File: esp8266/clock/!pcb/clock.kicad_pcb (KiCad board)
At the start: 2 copper layers, 45.2 x 57 mm, 17 parts, among them J1 GPIO, U3 BME280, U4 OLED, U5 LED, U6 SPARE

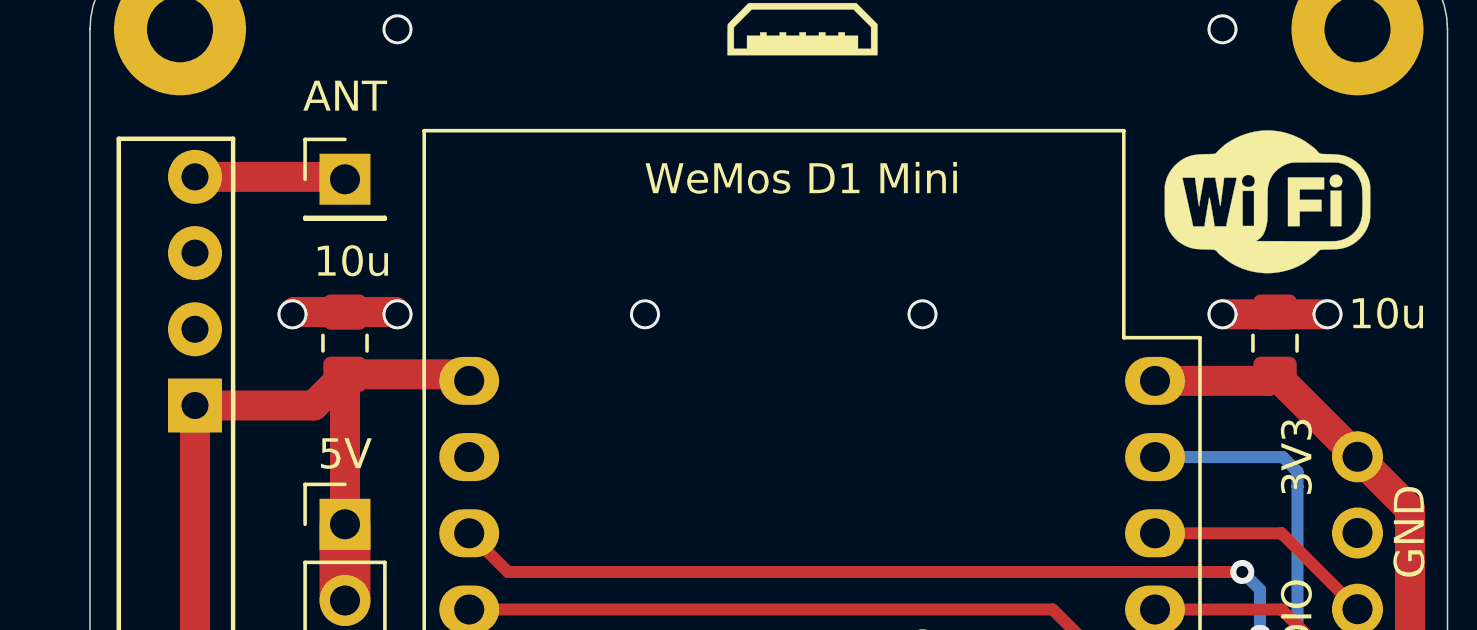
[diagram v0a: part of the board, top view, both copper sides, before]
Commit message: clock: Almost ready
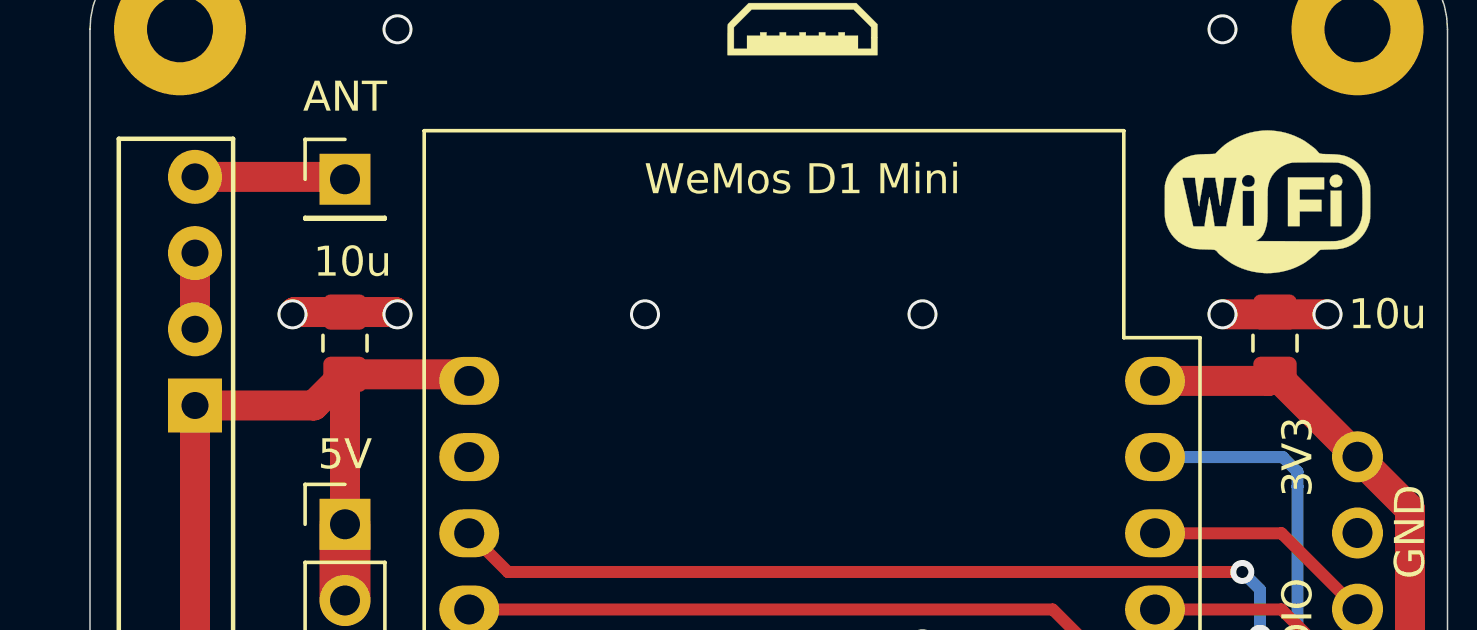
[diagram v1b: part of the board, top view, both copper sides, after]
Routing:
- net GND: track 13.1 -> 15.6 mm
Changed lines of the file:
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@@
     (thickness 1.6)
     (drawings 23)
-    (tracks 111)
+    (tracks 112)
     (zones 0)
     (modules 17)
@@
       (outputformat 1)
       (mirror false)
-      (drillshape 1)
+      (drillshape 0)
       (scaleselection 1)
-      (outputdirectory ""))
+      (outputdirectory "gerbs/"))
   )
   (net 0 "")
@@
       (effects (font (size 0.5 0.5) (thickness 0.08)))
     )
-    (pad 1 smd roundrect (at -1.0375 0 90) (size 1.175 1.45) (layers F.Cu F.Paste F.Mask) (roundrect_rratio 0.212766)
+    (pad 1 smd roundrect (at -1.0375 0 90) (size 1.175 1.45) (layers F.Cu F.Paste F.Mask) (roundrect_rratio 0.2127659574468085)
       (net 1 +5V))
-    (pad 2 smd roundrect (at 1.0375 0 90) (size 1.175 1.45) (layers F.Cu F.Paste F.Mask) (roundrect_rratio 0.212766)
+    (pad 2 smd roundrect (at 1.0375 0 90) (size 1.175 1.45) (layers F.Cu F.Paste F.Mask) (roundrect_rratio 0.2127659574468085)
       (net 2 GND))
     (model ${KISYS3DMOD}/Capacitor_SMD.3dshapes/C_0805_2012Metric.wrl
@@
       (effects (font (size 0.5 0.5) (thickness 0.08)))
     )
-    (pad 2 smd roundrect (at 1.0375 0 270) (size 1.175 1.45) (layers F.Cu F.Paste F.Mask) (roundrect_rratio 0.212766)
+    (pad 2 smd roundrect (at 1.0375 0 270) (size 1.175 1.45) (layers F.Cu F.Paste F.Mask) (roundrect_rratio 0.2127659574468085)
       (net 3 +3V3))
-    (pad 1 smd roundrect (at -1.0375 0 270) (size 1.175 1.45) (layers F.Cu F.Paste F.Mask) (roundrect_rratio 0.212766)
+    (pad 1 smd roundrect (at -1.0375 0 270) (size 1.175 1.45) (layers F.Cu F.Paste F.Mask) (roundrect_rratio 0.2127659574468085)
       (net 2 GND))
     (model ${KISYS3DMOD}/Capacitor_SMD.3dshapes/C_0805_2012Metric.wrl
@@
   (via (at 56.75 85.5) (size 1) (drill 0.8) (layers F.Cu B.Cu) (net 2))
   (via (at 57.25 109.5) (size 1) (drill 0.8) (layers F.Cu B.Cu) (net 2))
+  (segment (start 54 71.46) (end 54 74) (width 1) (layer F.Cu) (net 2))
   (segment (start 84.772808 109) (end 78.04 109) (width 1) (layer F.Cu) (net 3))
   (segment (start 94.500001 80.000001) (end 94.500001 87.749999) (width 1) (layer F.Cu) (net 3))
